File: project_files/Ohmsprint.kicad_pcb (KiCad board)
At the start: 2 copper layers, 150 x 150 mm, 122 parts, among them J2 MEM2067-02-180-00-A, J3 PJ-002AH-SMT-TR, J4 SJ-3523-SMT-TR, J5 541324062, J6 USB4110-GF-A, Q1 SS8050, Q2 SS8050, Q3 AO3400A, SW1 SW_Push_1_Red, SW2 SW_Push_1_Red, SW3 SW_Push_2_Blue, U1 ESP32-WROOM-32E-N4, U2 AP63203WU, U3 AP63200WU, U4 ATM90E26-YU, U5 ABS210-13, U6 CP2102N-A02-GQFN28R, U7 MCP1727-3302E/SN, U8 TPS2121RUXR, Y1 ABLS-8.192MHZ-B2-T

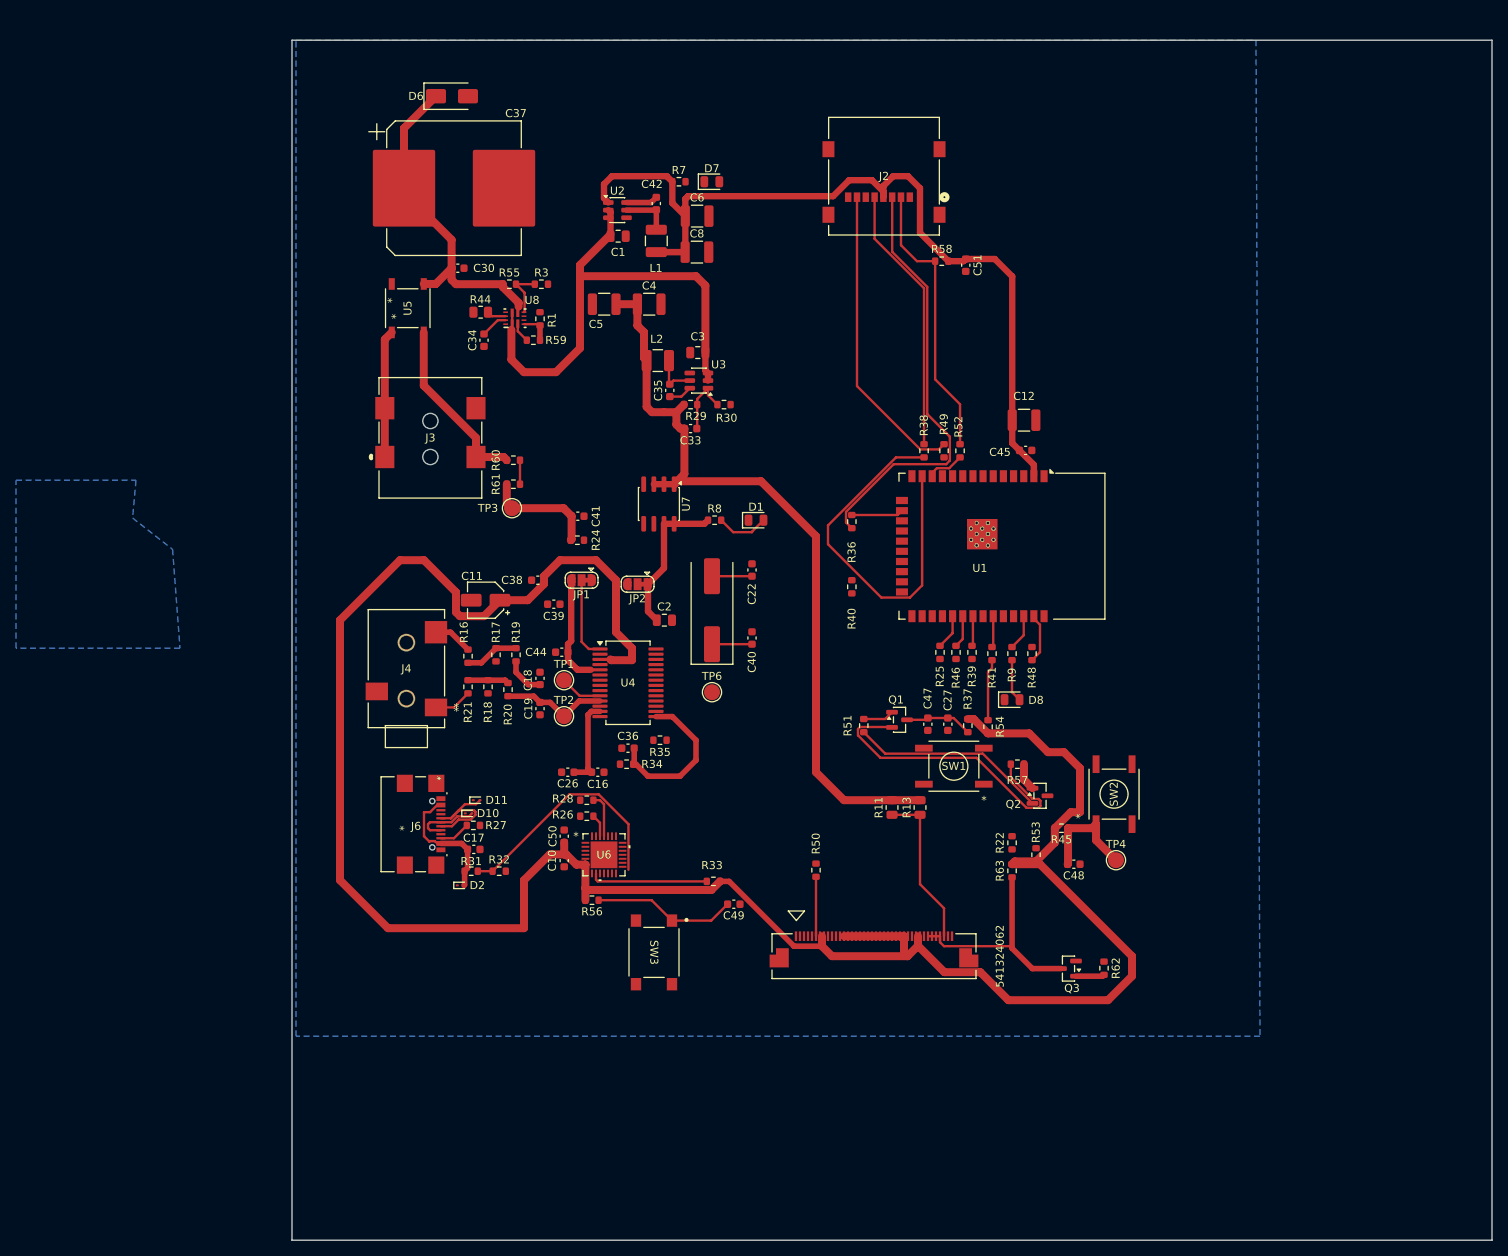
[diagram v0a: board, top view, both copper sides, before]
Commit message: Uradjen PCB
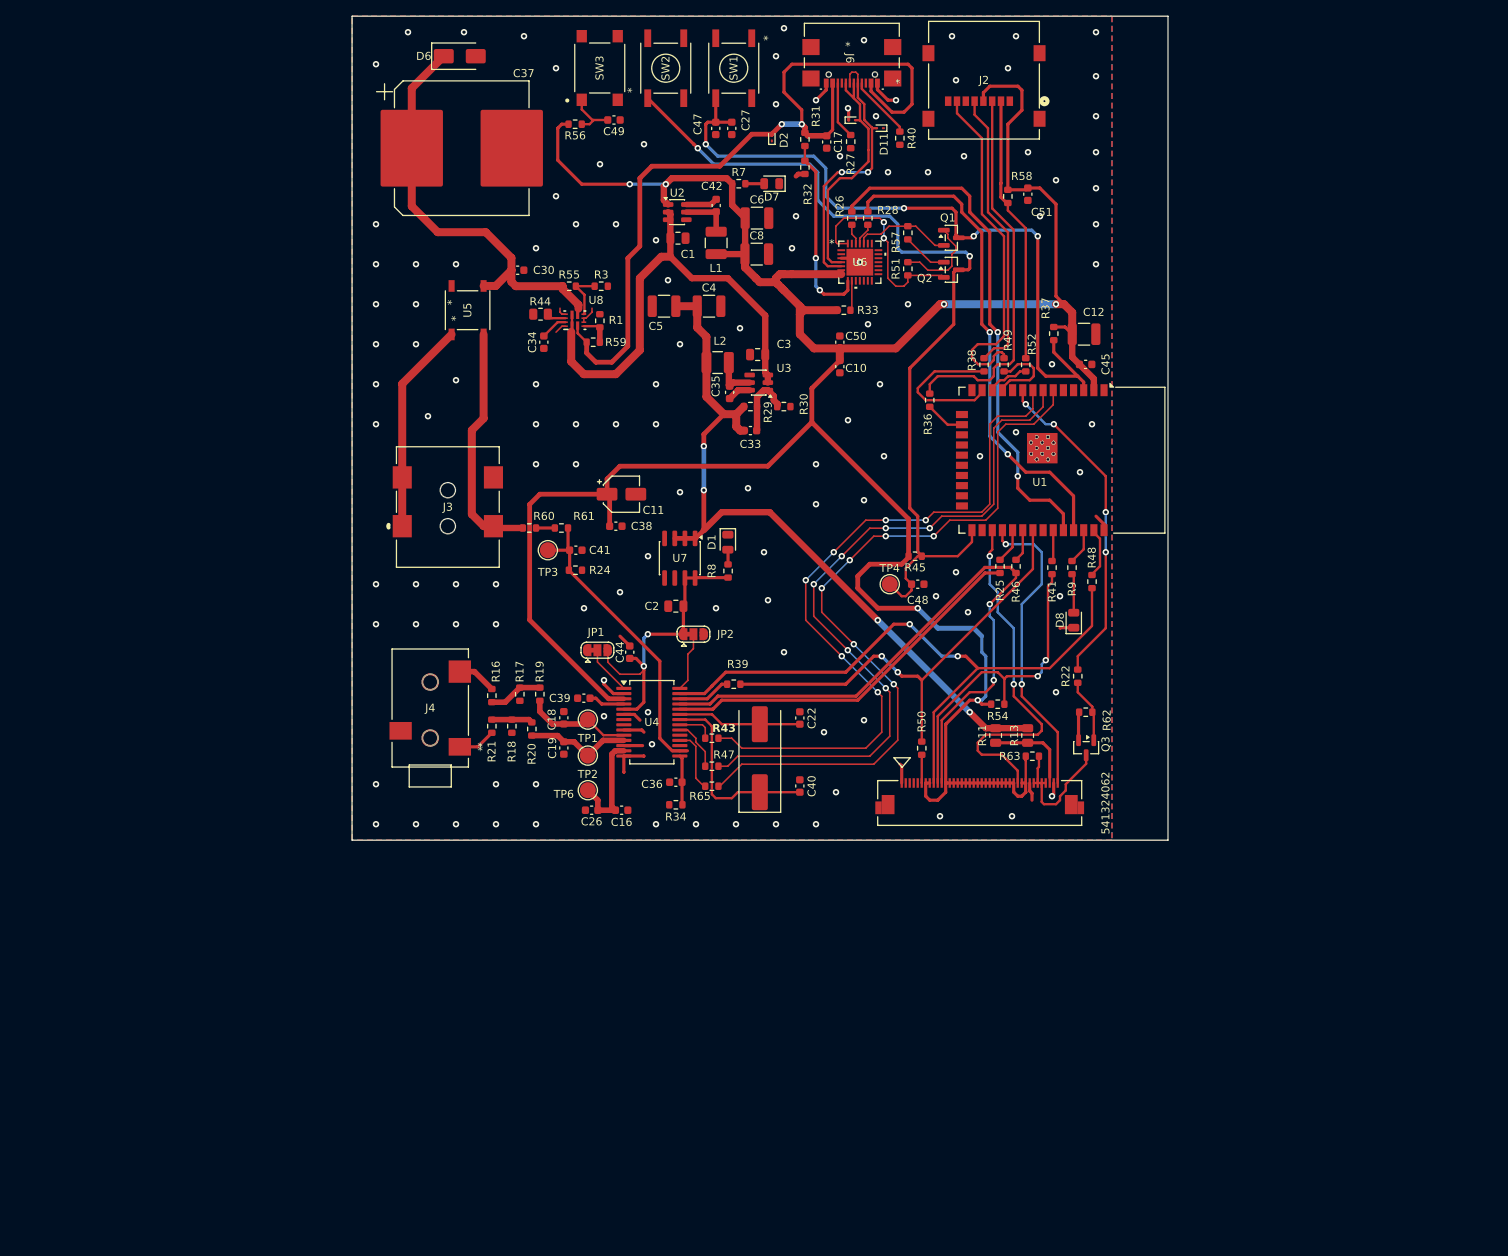
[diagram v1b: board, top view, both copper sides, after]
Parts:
- removed R35: 0R, Resistor_SMD:R_0603_1608Metric
- removed R53: 10k, Resistor_SMD:R_0603_1608Metric
- added R43: 33R, Resistor_SMD:R_0603_1608Metric, F.Cu at (72.0, 104.2)
- added R47: 33R, Resistor_SMD:R_0603_1608Metric, F.Cu at (72.0, 107.8)
- added R65: 33R, Resistor_SMD:R_0603_1608Metric, F.Cu at (72.0, 110.2)
- moved SW3 110.8 mm to (58.0, 20.5), turned to 90 degrees
- moved J6 110.5 mm to (89.5, 19.0), turned to 180 degrees
- moved SW2 106.7 mm to (66.2, 20.5)
- moved D2 101.2 mm to (79.5, 29.2), turned to 90 degrees
- moved R31 100.5 mm to (83.6, 29.4), turned to -90 degrees
- moved C49 99.2 mm to (59.7, 27.0)
- moved D10 99.0 mm to (89.5, 27.0)
- moved C17 98.8 mm to (86.3, 29.7), turned to -90 degrees
- moved D11 98.0 mm to (93.0, 28.0), turned to 180 degrees
- moved R27 97.6 mm to (89.3, 29.7), turned to -90 degrees
- moved R56 97.0 mm to (54.9, 27.5)
- moved R32 95.9 mm to (83.6, 32.9), turned to -90 degrees
- moved SW1 91.5 mm to (74.7, 20.5), turned to 90 degrees
- moved R26 81.8 mm to (89.5, 39.2), turned to 90 degrees
- moved R28 80.8 mm to (91.5, 39.2), turned to 90 degrees
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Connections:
- C16 pad 2: GNDA -> GND
- C18 pad 2: GNDA -> GND
- C19 pad 1: GNDA -> GND
- C26 pad 2: GNDA -> GND
- C36 pad 2: GNDA -> GND
- C41 pad 2: GNDA -> GND
- C44 pad 1: GNDA -> GND
- R17 pad 2: GNDA -> GND
- R18 pad 1: GNDA -> GND
- R24 pad 1: GNDA -> GND
- R34 pad 1: GNDA -> GND
- U1 pad 26: /random -> unconnected-(U1-IO4-Pad26)
- U4 pad 14: GNDA -> GND
- U4 pad 18: /ATIM_CF1 -> Net-(U4-CF1)
- U4 pad 20: /ATM_IRQ -> Net-(U4-IRQ)
- U4 pad 21: /ATM_ZX -> Net-(U4-ZX)
- U4 pad 6: GNDA -> GND
- U4 pad 7: GNDA -> GND
- U4 pad 8: GNDA -> GND
- U6 pad 4: /Data+ -> /D+
- U6 pad 5: /Data- -> /D-
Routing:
- net /IO0: track 13.8 -> 112.2 mm, vias 0 -> 2
- net /ATM_CF1: track 0.00 -> 93.5 mm, vias 0 -> 6
- net /ATM_IRQ: track 0.00 -> 91.4 mm, vias 0 -> 6
- net /ATM_ZX: track 0.00 -> 90.2 mm, vias 0 -> 6
- net VBUS: track 18.9 -> 102.2 mm, vias 0 -> 2
- net /EN: track 8.43 -> 89.6 mm, vias 0 -> 4
- net /SCLK: track 0.00 -> 81.1 mm, vias 0 -> 2
- net /MOSI: track 0.00 -> 80.9 mm, vias 0 -> 2
- net /RXD0: track 0.00 -> 64.8 mm, vias 0 -> 2
- net /TXD0: track 0.00 -> 61.9 mm, vias 0 -> 2
- net /MISO: track 3.75 -> 57.5 mm, vias 0 -> 2
- net +3.3VD: track 392.9 -> 344.7 mm, vias 0 -> 6
- net GND: track 0.00 -> 47.7 mm, vias 0 -> 43
- net /ATM_CS: track 0.00 -> 47.1 mm
- net /DSP_RESX: track 0.00 -> 45.1 mm, vias 0 -> 2
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- added copper zone on F.Cu, net GND
- removed copper zone on B.Cu, net GNDA
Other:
- board size 150 x 150 mm -> 102 x 103 mm
